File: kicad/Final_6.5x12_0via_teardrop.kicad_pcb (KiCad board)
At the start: 2 copper layers, 33.6 x 17.7 mm, 18 parts, among them J3 FDTI, SW1 SW_Push, U1 ATmega328P-A

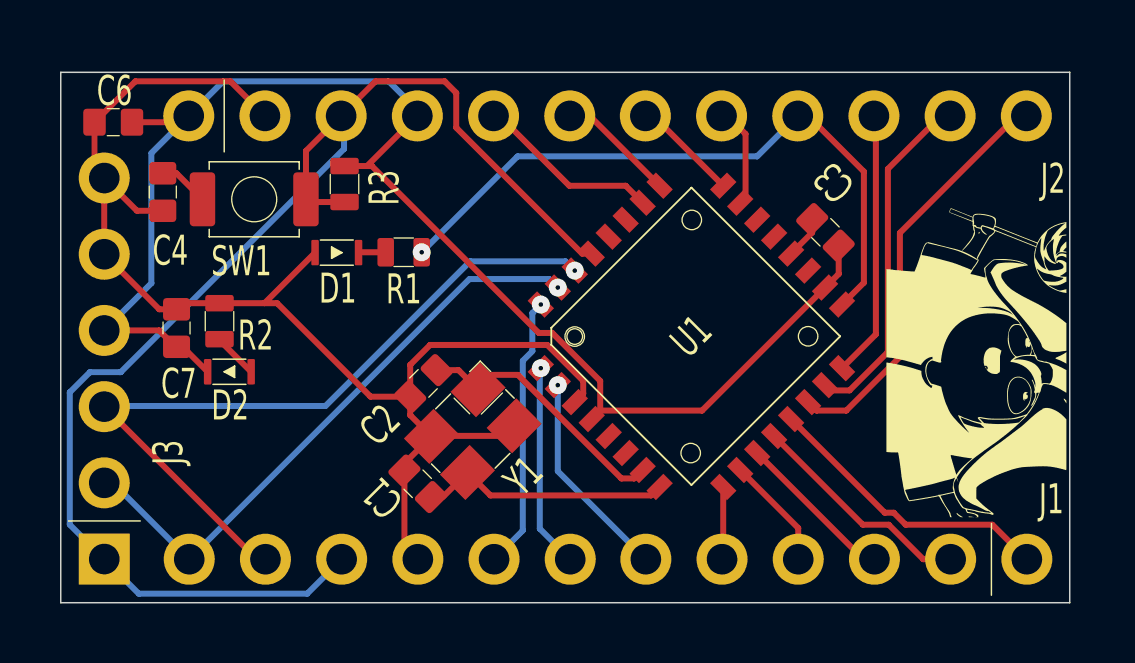
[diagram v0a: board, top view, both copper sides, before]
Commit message: Done ig
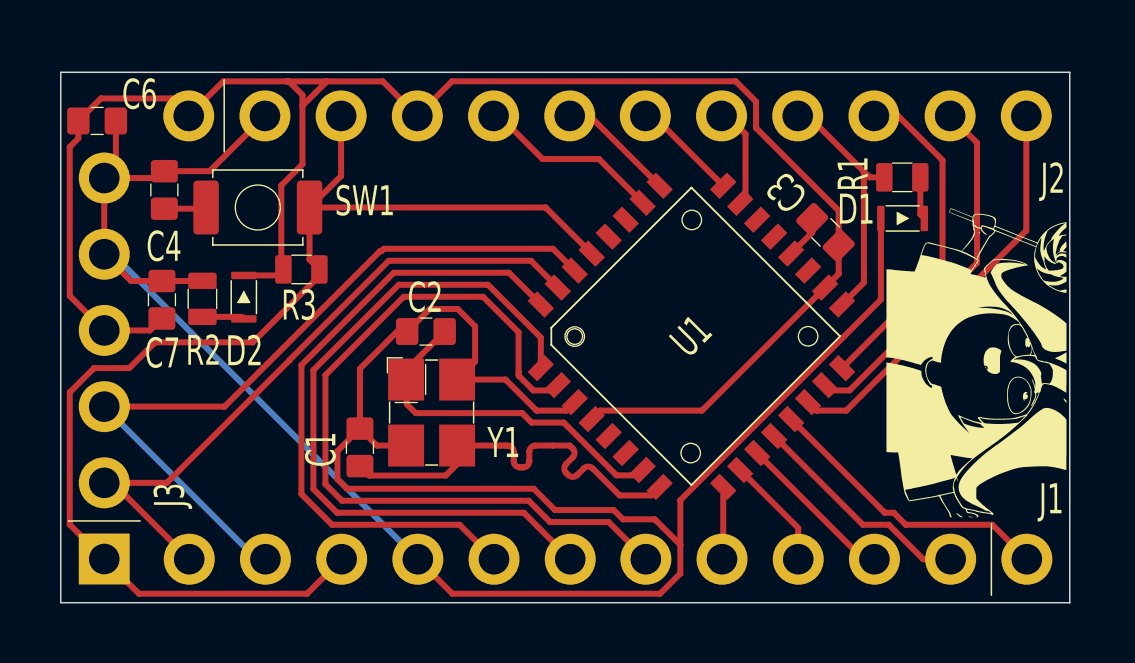
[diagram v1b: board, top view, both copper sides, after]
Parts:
- moved D1 18.9 mm to (77.5, 92.6)
- moved R1 16.8 mm to (77.5, 91.2), turned to 0 degrees
- moved R3 3.19 mm to (57.5, 94.3), turned to 0 degrees
- moved D2 2.53 mm to (55.6, 95.2), turned to 90 degrees
- moved C1 2.28 mm to (59.5, 100.2), turned to 90 degrees
- moved C2 1.73 mm to (61.6, 96.3), turned to 180 degrees
- moved Y1 1.51 mm to (61.8, 99.0), turned to -90 degrees
- moved C7 1.06 mm to (52.9, 95.3)
- moved R2 0.94 mm to (54.2, 95.2)
- moved C6 0.54 mm to (50.7, 89.3), turned to 0 degrees
- moved SW1 0.30 mm to (56.0, 92.2)
- moved C4 0.09 mm to (52.9, 91.6), turned to -90 degrees
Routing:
- net GND: track 45.2 -> 83.9 mm
- net D4: track 7.02 -> 26.7 mm, vias 1 -> 0
- net D3: track 6.47 -> 24.0 mm, vias 1 -> 0
- net SCK: track 22.4 -> 8.58 mm, vias 1 -> 0
- net D2: track 9.14 -> 21.3 mm, vias 1 -> 0
- net RAW: track 49.2 -> 61.0 mm
- net Net-(U1-XTAL2/PB7): track 8.00 -> 14.7 mm
- net DTR: track 45.1 -> 41.1 mm
- net Net-(U1-XTAL1/PB6): track 8.89 -> 12.5 mm
- net TXO: track 20.2 -> 22.7 mm, vias 1 -> 0
- net MISO: track 9.37 -> 11.2 mm
- net RXI: track 25.3 -> 26.0 mm, vias 1 -> 0
- net Net-(D1-Pad2): track 0.89 -> 1.43 mm
